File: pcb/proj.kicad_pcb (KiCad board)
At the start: 2 copper layers, 125 x 185 mm, 150 parts, among them J1 Conn_02x05_Odd_Even, Q1 MMBT3904, SW1 Reset, SW10 8, SW11 9, SW12 /, SW13 Deg/Rad, SW14 Clear, SW15 4, SW16 5, SW17 6, SW18 X, SW19 Constants, SW2 Y/Stats, SW20 Del, SW21 1, SW22 2, SW23 3, SW24 -, SW25 Alpha, SW26 (/), SW27 Sin(x)/Sin-1(x), SW28 Cos(x)/Cos-1(x), SW29 Tan(x)/Tan-1(x), SW3 ./,, SW30 +, SW31 2nd, SW32 Γ(x), SW33 x^y/y√x, SW34 x^2/√x, SW35 log(x)/ln(x), SW36 e^x/10^x, SW37 Graph, SW38 Programs, SW39 Left, SW4 0, SW40 Up, SW41 Right, SW42 Down, SW43 Power, SW44 FPU BOOT0, SW45 Reset, SW5 +/-, SW6 Solve/=, SW7 Sci/Norm, SW8 X/Matrix, SW9 7, U1 PIC16C74, U2 STM32F401RCTx, U3 74HC238, U4 ISL9111EH50Z-T7A, U5 SN74LVC1G32DBVR, U6 TPS61021A, U7 SiP32510DT, U8 SN74LV1T34DBV, Y1 20MHz

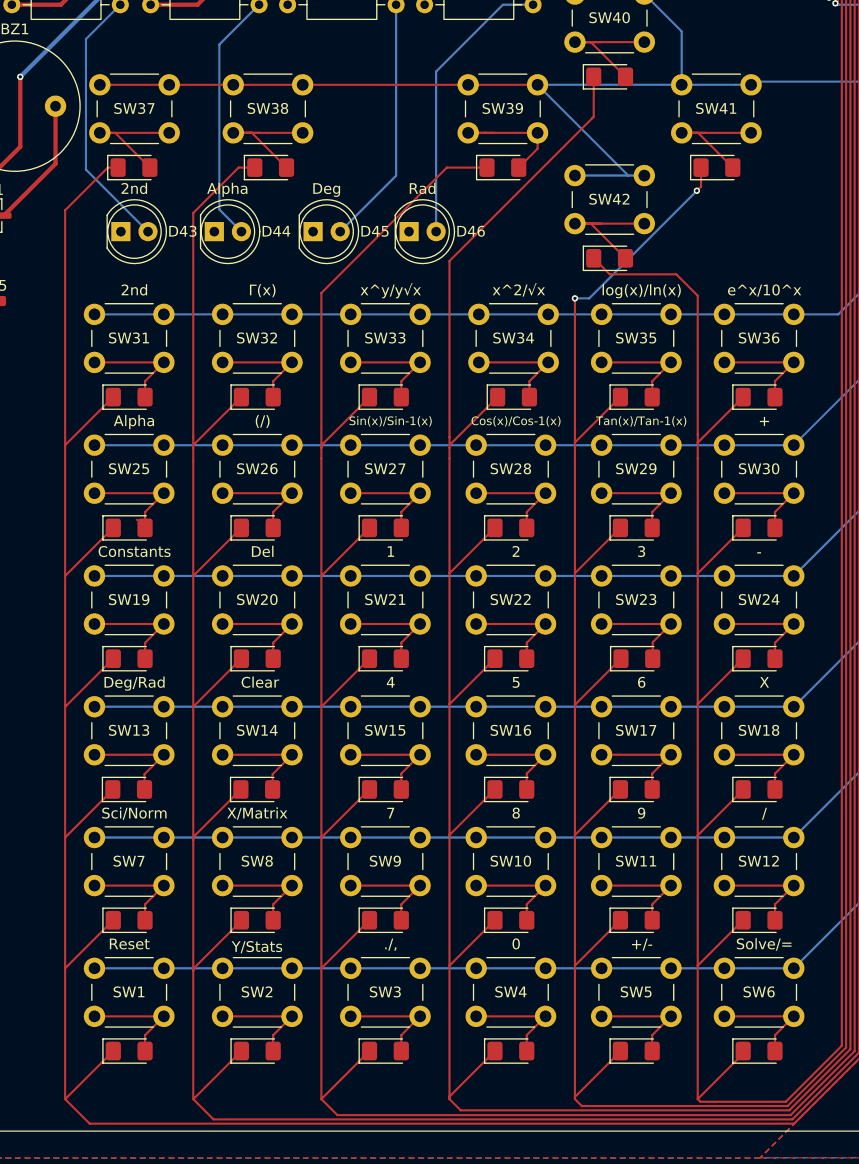
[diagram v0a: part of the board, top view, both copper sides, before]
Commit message: w
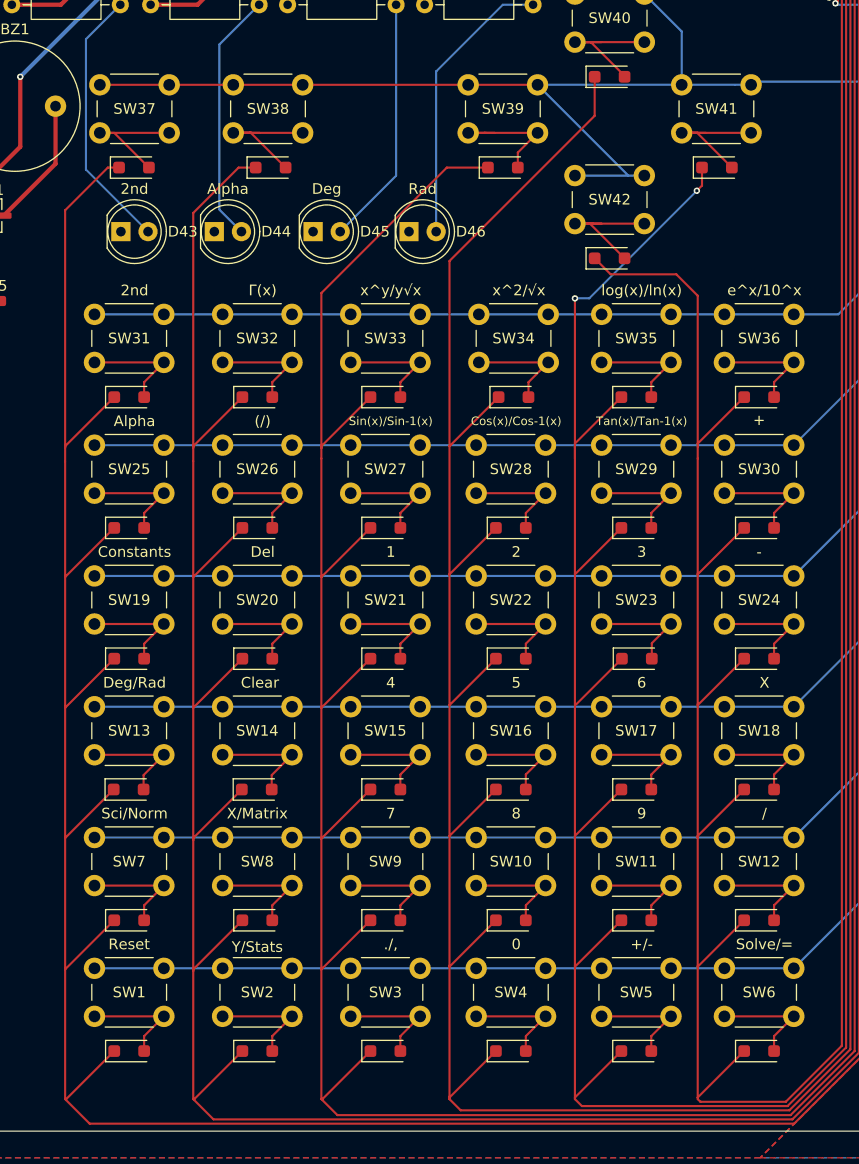
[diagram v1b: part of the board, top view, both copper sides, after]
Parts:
- D1, D10, D11, D12, D13, D14, D15, D16, D17, D18, D19, D2, D20, D21, D22, D23, D24, D25, D26, D27, D28, D29, D3, D30, D31, D32, D33, D34, D35, D36, D37, D38, D39, D4, D40, D41, D42, D5, D6, D7, D8, D9: footprint Diode_SMD:D_1206_3216Metric_Pad1.42x1.75mm_HandSolder -> Diode_SMD:D_SOD-123F
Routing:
- net Net-(D11-K): track 339.3 -> 341.4 mm
- net Net-(D38-A): track 15.5 -> 17.2 mm
- net Net-(D41-A): track 14.9 -> 16.4 mm
- net Net-(D42-A): track 15.3 -> 16.7 mm
- net Net-(D15-K): track 364.1 -> 365.2 mm
- net Net-(D14-K): track 369.1 -> 370.0 mm
- net Net-(D10-K): track 357.7 -> 358.5 mm
- net Net-(D1-K): track 378.3 -> 379.1 mm
- net Net-(D12-K): track 323.2 -> 323.8 mm
